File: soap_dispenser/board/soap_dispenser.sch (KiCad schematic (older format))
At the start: 48 parts, among them M1 Motor_DC, Q1 DMG2305UX, Q11 MMBT4401, Q2 DMG3420U, Q3 DMG2305UX, Q4 DMG3420U, Q5 MMBT4401, SW1 SW_SPDT, SW8 SW_Push, U1 ATtiny48-AU

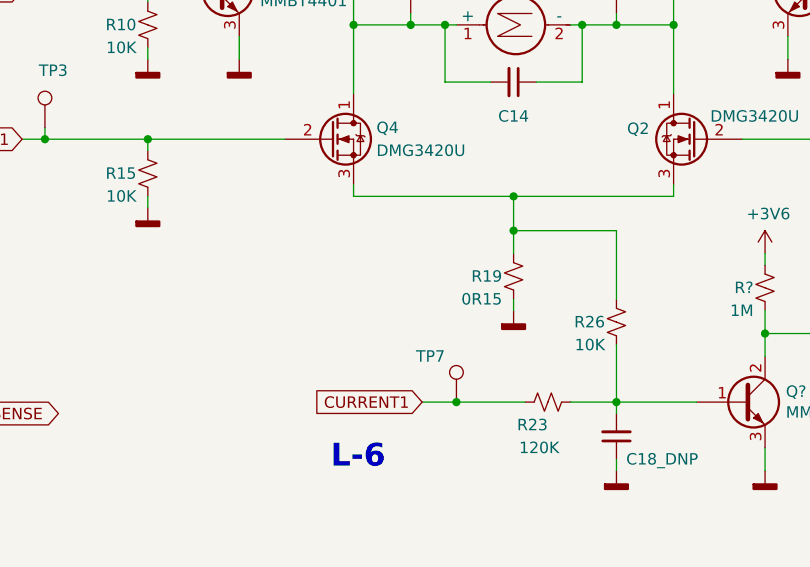
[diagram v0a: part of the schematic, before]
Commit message: Added a comment with current sense resistor package size.
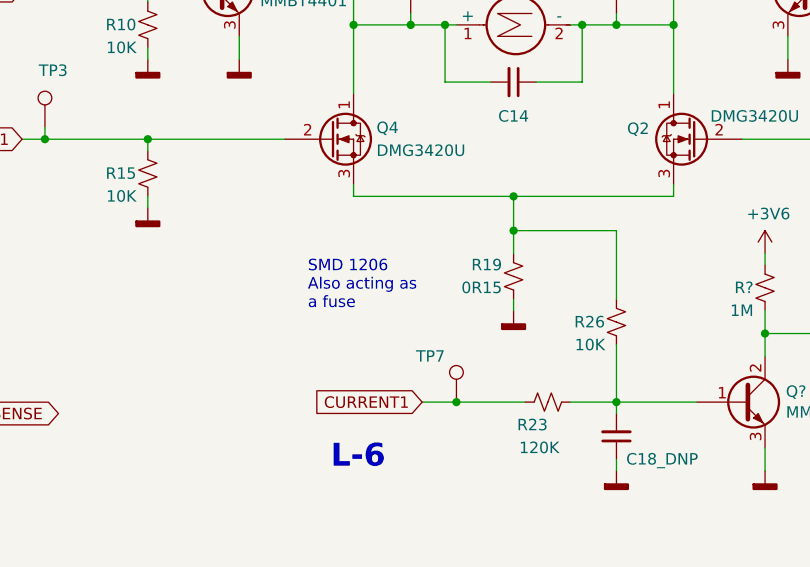
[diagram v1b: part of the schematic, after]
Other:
- note added: "SMD 1206\nAlso acting as \na fuse"
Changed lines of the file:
@@
 U 1 1 5C10B5B4
 P 7550 3050
-F 0 "R19" H 7600 3050 50  0000 L CNN
-F 1 "0R15" H 7600 3150 50  0000 L CNN
+F 0 "R19" H 7600 3000 50  0000 L CNN
+F 1 "0R15" H 7600 3100 50  0000 L CNN
 F 2 "" H 7550 3050 50  0001 C CNN
 F 3 "~" H 7550 3050 50  0001 C CNN
@@
 	1    0    0    -1
 $EndComp
+Text Notes 6650 3200 0    50   ~ 0
+SMD 1206\nAlso acting as \na fuse
 $EndSCHEMATC
